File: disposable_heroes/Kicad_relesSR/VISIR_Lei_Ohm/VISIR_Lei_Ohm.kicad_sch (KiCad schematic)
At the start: 24 parts, among them J1 Raspberry PI5, J2 Fonte dc, J3 Fonte 12V, J4 Fonte 5V, K1 3572-1220-123, K2 3572-1220-123, K3 3572-1220-123, K4 3570-1331-123, K5 3570-1331-123, K6 3570-1331-123, K7 3570-1331-123, K8 3570-1331-123, K9 3570-1331-123, U1 74HC595N_112, U2 ULN2003, U3 ULN2003, U4 74HC595N_112

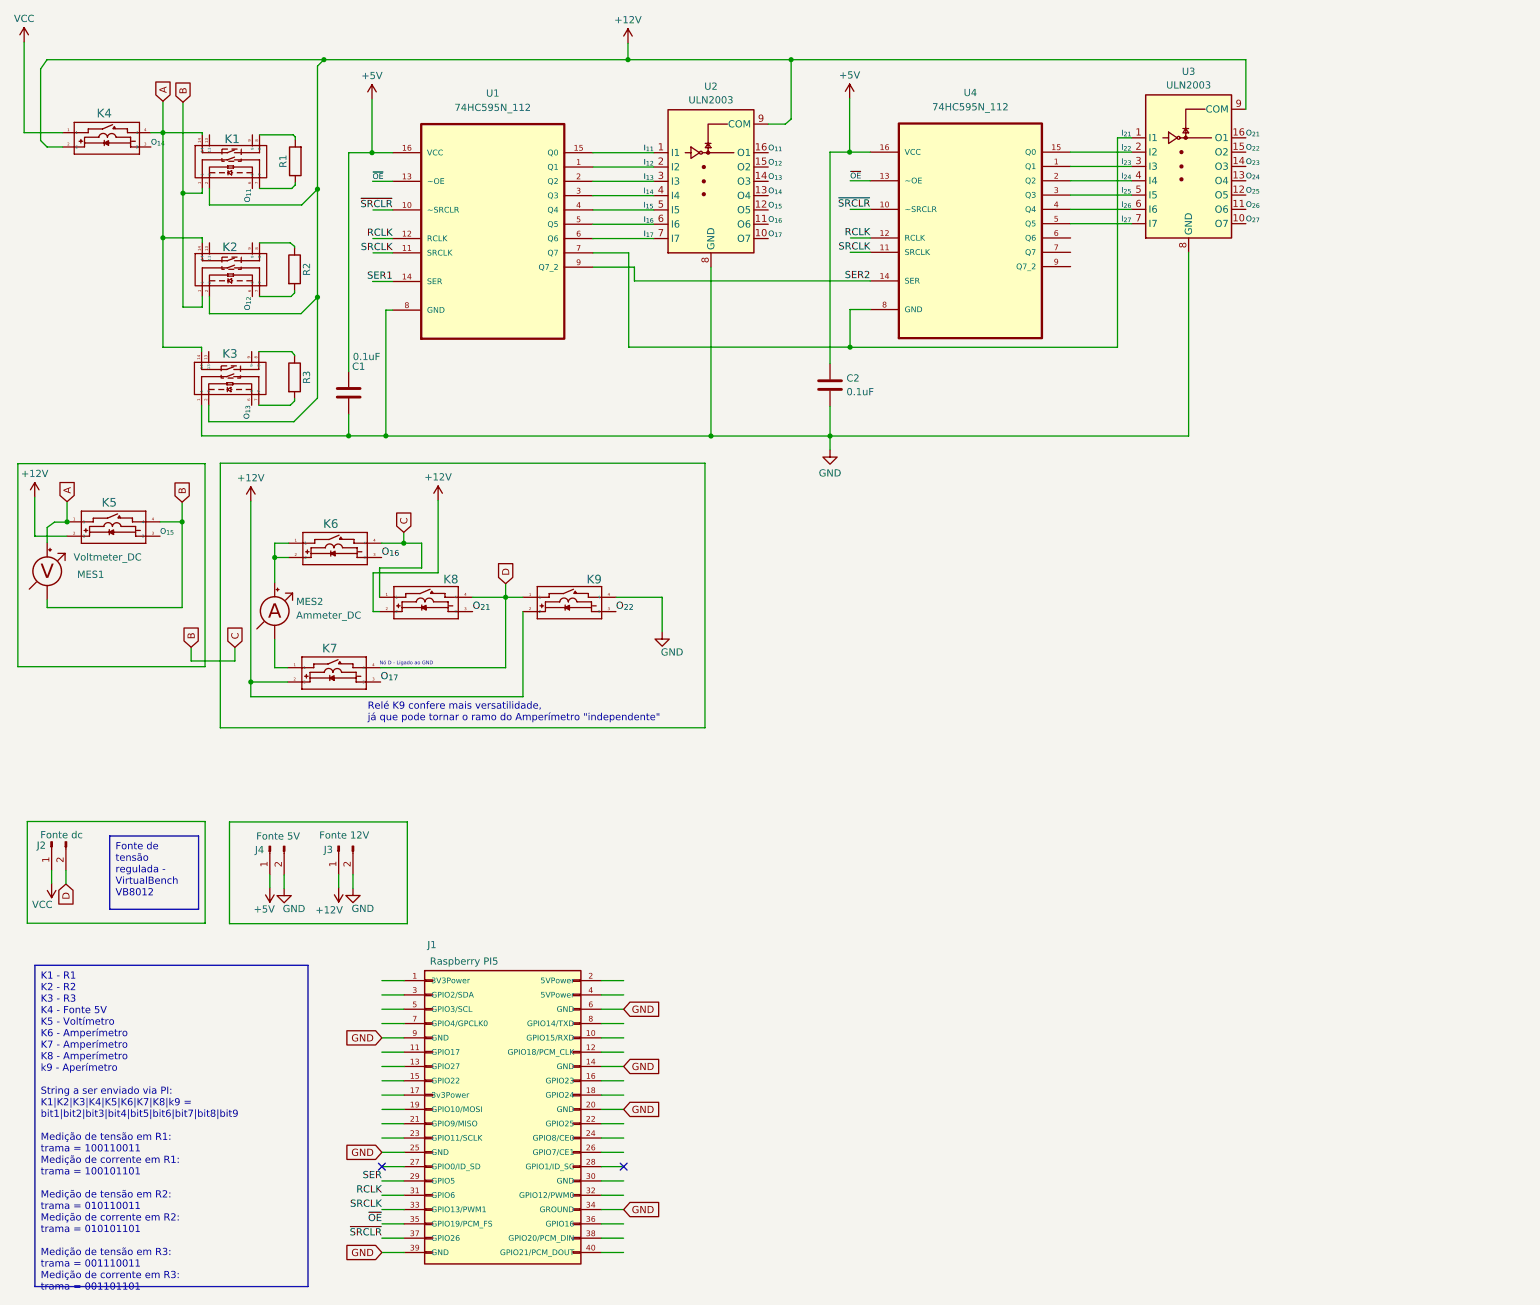
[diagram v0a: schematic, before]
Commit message: update
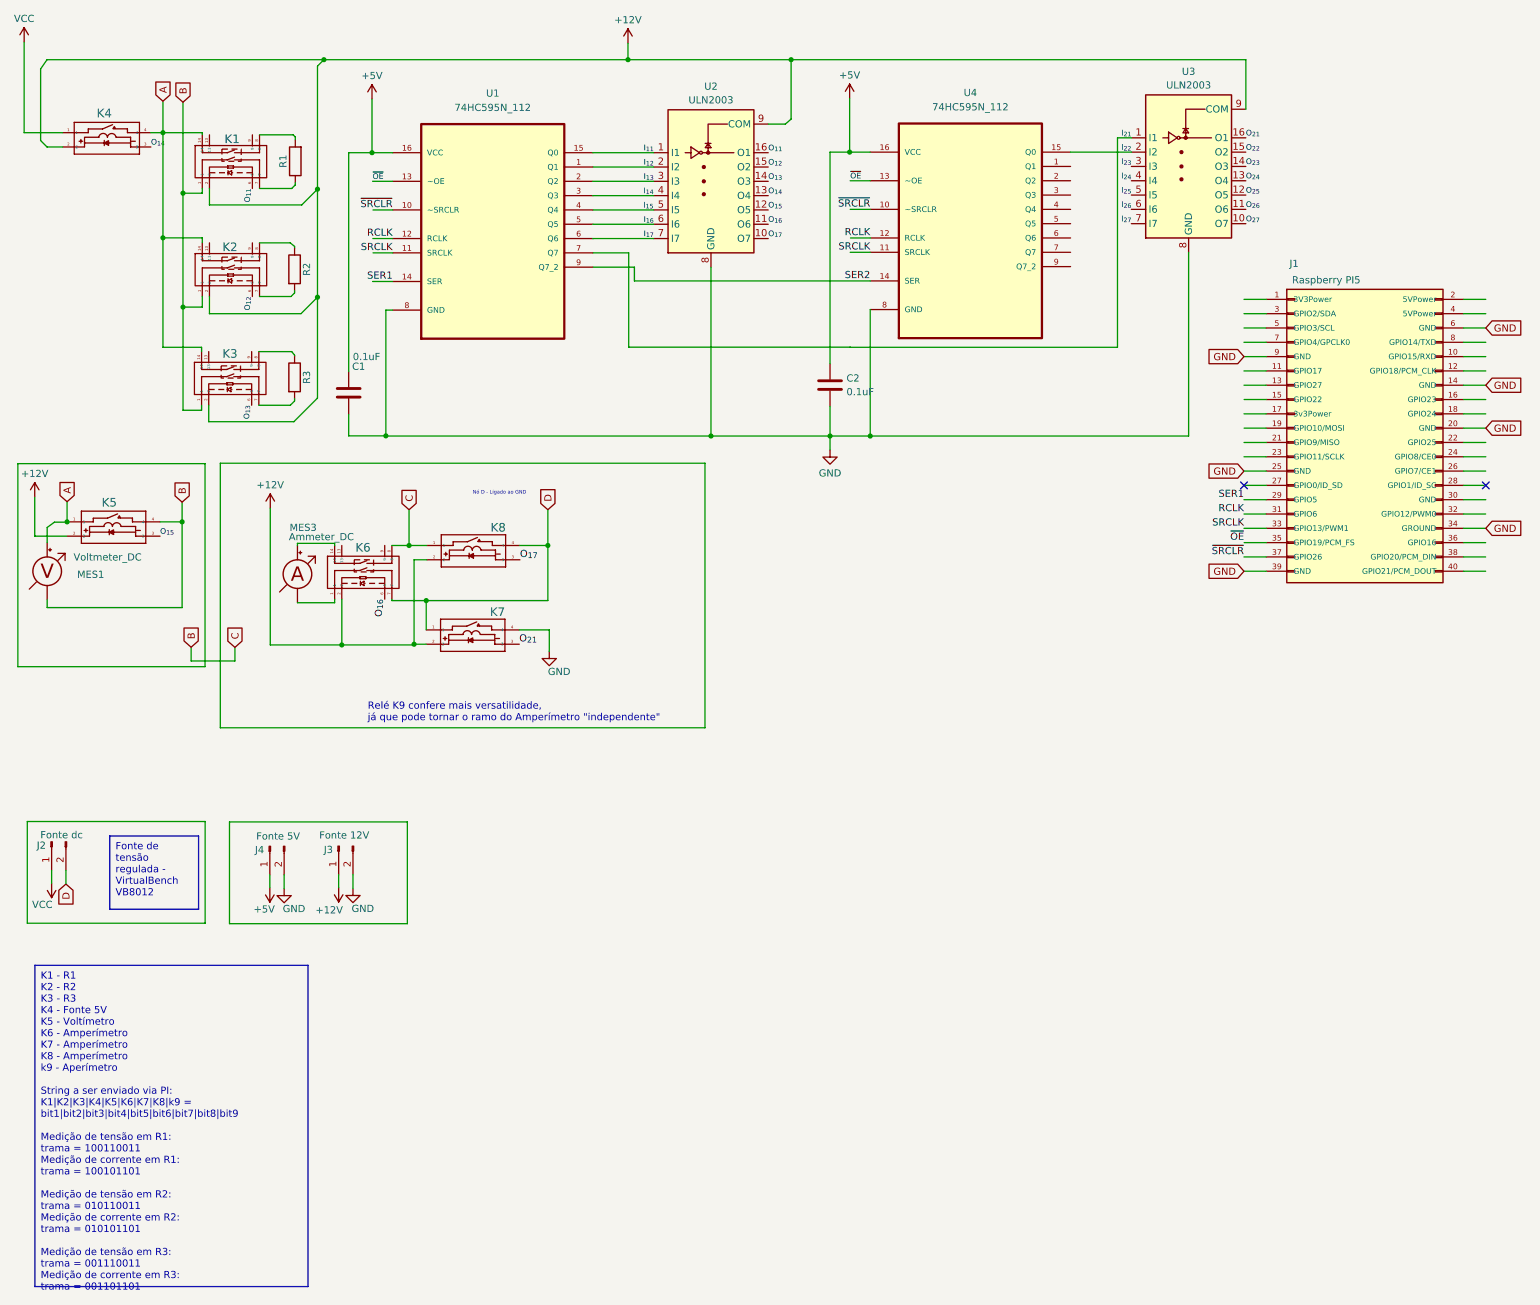
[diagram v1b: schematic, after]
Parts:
- removed K6, K9: 3570-1331-123, 3570-1220-123:SIP_3570-1331_COM, symbol 3570-1331-123:3570-1331-123
- removed MES2: Ammeter_DC, Connector_PinHeader_2.54mm:PinHeader_1x02_P2.54mm_Vertical, symbol Device:Ammeter_DC
- added K6: 3572-1220-123, 3572-1220-053:RELAY8_3572-1220-053_COM, symbol 3572-1220-123:3572-1220-123
- added MES3: Ammeter_DC, Connector_PinHeader_2.54mm:PinHeader_1x02_P2.54mm_Vertical, symbol Device:Ammeter_DC
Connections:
- net SER is gone; now on net SER1: J1.29 (GPIO5)
- net +12V: now also K6.2
- net B: now also K3.1, K6.8
- net D: now also K7.1, K6.7; no longer K7.4
- net GND: now also K7.4, U4.8 (GND); no longer K3.1
- net I_{21}: no longer U4.8 (GND)
- net I_{23}: no longer U4.1 (Q1)
- net I_{24}: no longer U4.2 (Q2)
- net I_{25}: no longer U4.3 (Q3)
- net I_{26}: no longer U4.4 (Q4)
- net I_{27}: no longer U4.5 (Q5)
- net O_{16}: now also K6.6
- net O_{17}: now also K8.3; no longer K7.3
- net O_{21}: now also K7.3; no longer K8.3
- new net: K6.1, MES3.1 (-)
- new net: K6.14, MES3.2 (+)
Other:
- moved on the sheet: J1
